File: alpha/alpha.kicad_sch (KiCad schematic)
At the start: 2 parts, among them M1 Motor_AC_3_phase

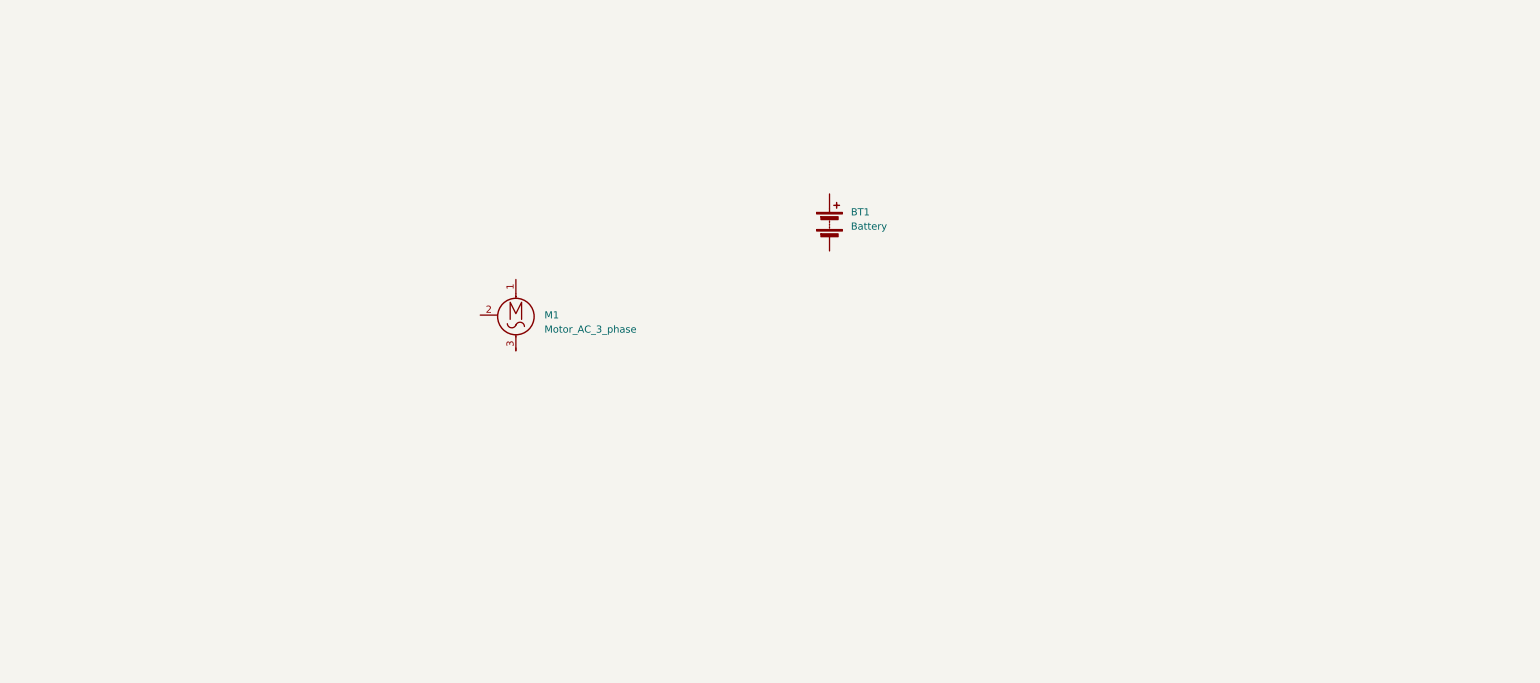
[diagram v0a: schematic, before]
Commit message: add power circuitry
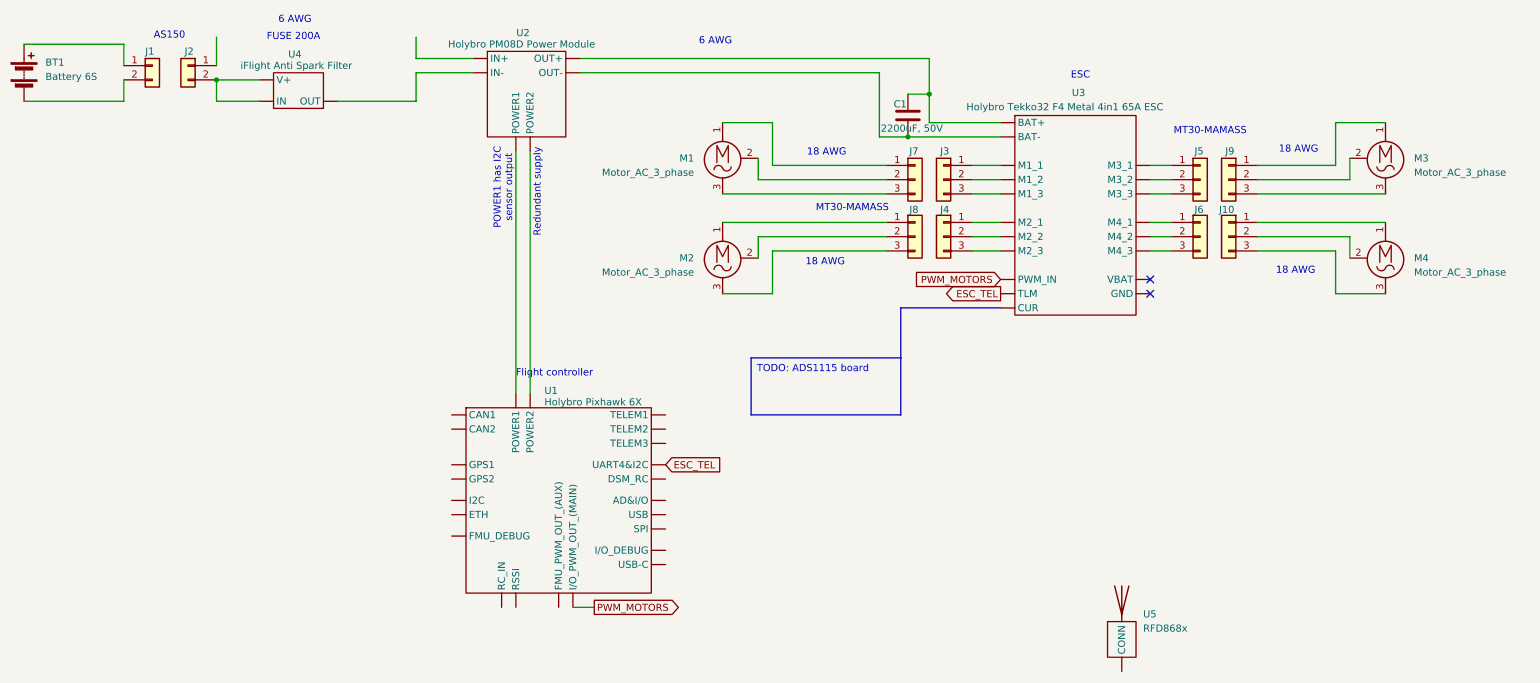
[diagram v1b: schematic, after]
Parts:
- added C1: 2200uF, 50V, symbol Device:C
- added J1, J2: Conn_01x02, symbol Connector_Generic:Conn_01x02
- added J10, J3, J4, J5, J6, J7, J8, J9: Conn_01x03, symbol Connector_Generic:Conn_01x03
- added M2, M3, M4: Motor_AC_3_phase, symbol Motors:Motor_AC_3_phase
- added U1: Holybro Pixhawk 6X, symbol Flight_Controllers:Holybro_Pixhawk_6X
- added U2: Holybro PM08D Power Module, symbol Power_Modules:Holybro_PM08D_Power_Module
- added U3: Holybro Tekko32 F4 Metal 4in1 65A ESC, symbol ESCs:Tekko32_F4_Metal_4in1_65A_ESC
- added U4: iFlight Anti Spark Filter, symbol Misc:iFlight_Anti_Spark_Filter
- added U5: RFD868x, symbol RF_Modules:RFD868x-EU_868Mhz_Long_Range
- BT1: value Battery -> Battery 6S
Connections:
- net at BT1.1 (+): now also J1.1 (Pin_1)
- net at BT1.2 (-): now also J1.2 (Pin_2)
- net at M1.1: now also J7.1 (Pin_1)
- net at M1.2: now also J7.2 (Pin_2)
- net at M1.3: now also J7.3 (Pin_3)
- new net: J5.1 (Pin_1), U3. (VBAT)
- new net: J5.2 (Pin_2), U3. (VBAT)
- new net: J5.3 (Pin_3), U3. (VBAT)
- new net: J9.1 (Pin_1), M3.1
- new net: J9.2 (Pin_2), M3.2
- new net: J9.3 (Pin_3), M3.3
- new net: U1. (USB-C), U2. (POWER2) (x2)
- new net: J8.1 (Pin_1), M2.1
- new net: J8.2 (Pin_2), M2.2
- new net: J8.3 (Pin_3), M2.3
- new net: C1.1, U2. (POWER2), U3. (VBAT)
- new net: C1.2, U2. (POWER2), U3. (VBAT)
- new net: J2.2 (Pin_2), U4. (V+)
- new net: U2. (POWER2), U4. (V+)
- new net: J10.1 (Pin_1), M4.1
- new net: J10.2 (Pin_2), M4.2
- new net: J10.3 (Pin_3), M4.3
- new net: J3.1 (Pin_1), U3. (VBAT)
- new net: J3.2 (Pin_2), U3. (VBAT)
- new net: J3.3 (Pin_3), U3. (VBAT)
- new net: J4.1 (Pin_1), U3. (VBAT)
- new net: J4.2 (Pin_2), U3. (VBAT)
- new net: J4.3 (Pin_3), U3. (VBAT)
- new net: J6.1 (Pin_1), U3. (VBAT)
- new net: J6.2 (Pin_2), U3. (VBAT)
- new net: J6.3 (Pin_3), U3. (VBAT)
- new net ESC_TEL: U1. (USB-C), U3. (VBAT)
- new net PWM_MOTORS: U1. (USB-C), U3. (VBAT)
- no-connect marks 0 -> 2
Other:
- note added: "18 AWG"
- note added: "6 AWG"
- note added: "AS150"
- note added: "ESC"
- note added: "FUSE 200A"
- note added: "Flight controller"
- note added: "MT30-MAMASS"
- note added: "POWER1 has I2C sensor output"
- note added: "Redundant supply"
- moved on the sheet: BT1
